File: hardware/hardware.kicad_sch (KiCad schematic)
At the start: 0 parts

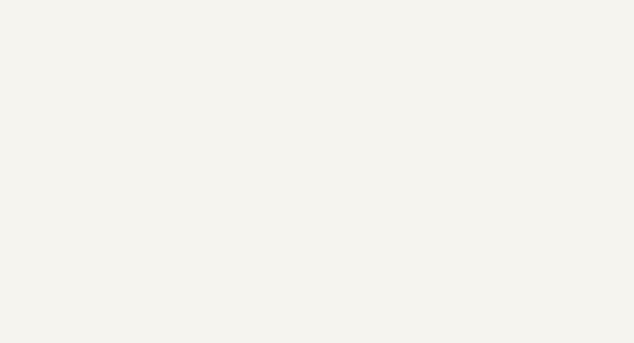
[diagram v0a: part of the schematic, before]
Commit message: update
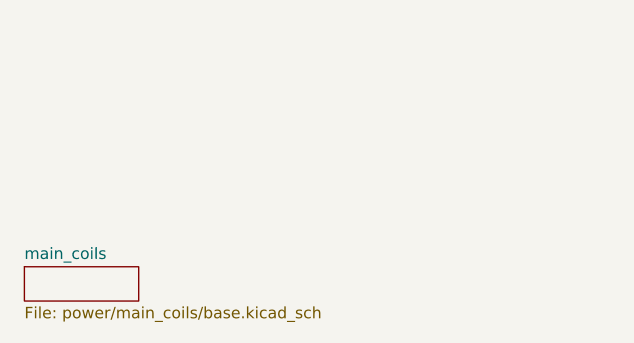
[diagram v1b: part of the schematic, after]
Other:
- added sheet main_coils (power/main_coils/base.kicad_sch)
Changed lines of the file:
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@@
 	(paper "A4")
+	(sheet
+		(at 36.195 168.91)
+		(size 12.7 3.81)
+		(exclude_from_sim no)
+		(in_bom yes)
+		(on_board yes)
+		(dnp no)
+		(fields_autoplaced yes)
+		(stroke
+			(width 0.1524)
+			(type solid)
+		)
+		(fill
+			(color 0 0 0 0.0000)
+		)
+		(property "Sheetname" "main_coils"
+			(at 36.195 168.1984 0)
+			(effects
+				(font
+					(size 1.27 1.27)
+				)
+				(justify left bottom)
+			)
+		)
+		(property "Sheetfile" "power/main_coils/base.kicad_sch"
+			(at 36.195 173.3046 0)
+			(effects
+				(font
+					(size 1.27 1.27)
+				)
+				(justify left top)
+			)
+		)
+		(instances
+			(project "hardware"
+				(path "/606d342f-174b-4504-b335-50f65aa4e733"
+					(page "13")
+				)
+			)
+		)
+	)
 	(sheet
 		(at 72.39 41.91)

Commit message: idk some changes
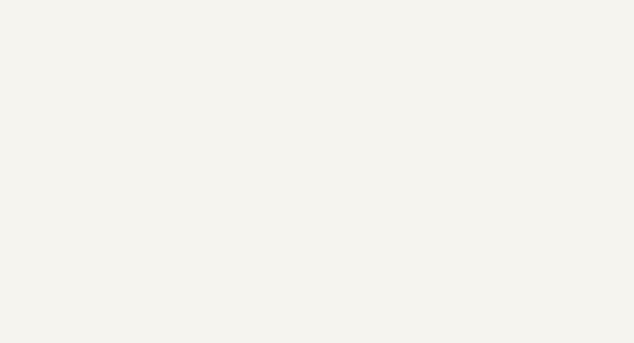
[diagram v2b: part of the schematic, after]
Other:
- removed sheet main_coils
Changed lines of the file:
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@@
 	(paper "A4")
-	(sheet
-		(at 36.195 168.91)
-		(size 12.7 3.81)
-		(exclude_from_sim no)
-		(in_bom yes)
-		(on_board yes)
-		(dnp no)
-		(fields_autoplaced yes)
-		(stroke
-			(width 0.1524)
-			(type solid)
-		)
-		(fill
-			(color 0 0 0 0.0000)
-		)
-		(property "Sheetname" "main_coils"
-			(at 36.195 168.1984 0)
-			(effects
-				(font
-					(size 1.27 1.27)
-				)
-				(justify left bottom)
-			)
-		)
-		(property "Sheetfile" "power/main_coils/base.kicad_sch"
-			(at 36.195 173.3046 0)
-			(effects
-				(font
-					(size 1.27 1.27)
-				)
-				(justify left top)
-			)
-		)
-		(instances
-			(project "hardware"
-				(path "/606d342f-174b-4504-b335-50f65aa4e733"
-					(page "13")
-				)
-			)
-		)
-	)
 	(sheet
 		(at 72.39 41.91)
